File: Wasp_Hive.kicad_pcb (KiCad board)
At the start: 2 copper layers, 132.8 x 172.5 mm, 157 parts, among them J0 WASP_OUT, J1 WASP_OUT, J10 WASP_OUT, J11 WASP_OUT, J12 WASP_OUT, J13 WASP_OUT, J14 WASP_OUT, J15 WASP_OUT, J16 DENS_OUT, J17 DENS_IN, J18 DROP_OUT, J19 PANIC_IN, J2 WASP_OUT, J20 GND, J21 GND, J22 GND, J23 GND, J24 GND, J25 PWR, J26 GND, J27 GND, J3 WASP_OUT, J4 WASP_OUT, J5 WASP_OUT, J6 WASP_OUT, J7 WASP_OUT, J8 WASP_OUT, J9 WASP_OUT, Q1 MMBT3904, Q2 MMBT3904, SW1 SW_SPDT, U0 74HC245, U1 74HC245, U2 MCP6002-xP, U3 MCP6002-xP, U4 TEENSY_3.2_MINIMAL, U5 L78M05ABDT-TR

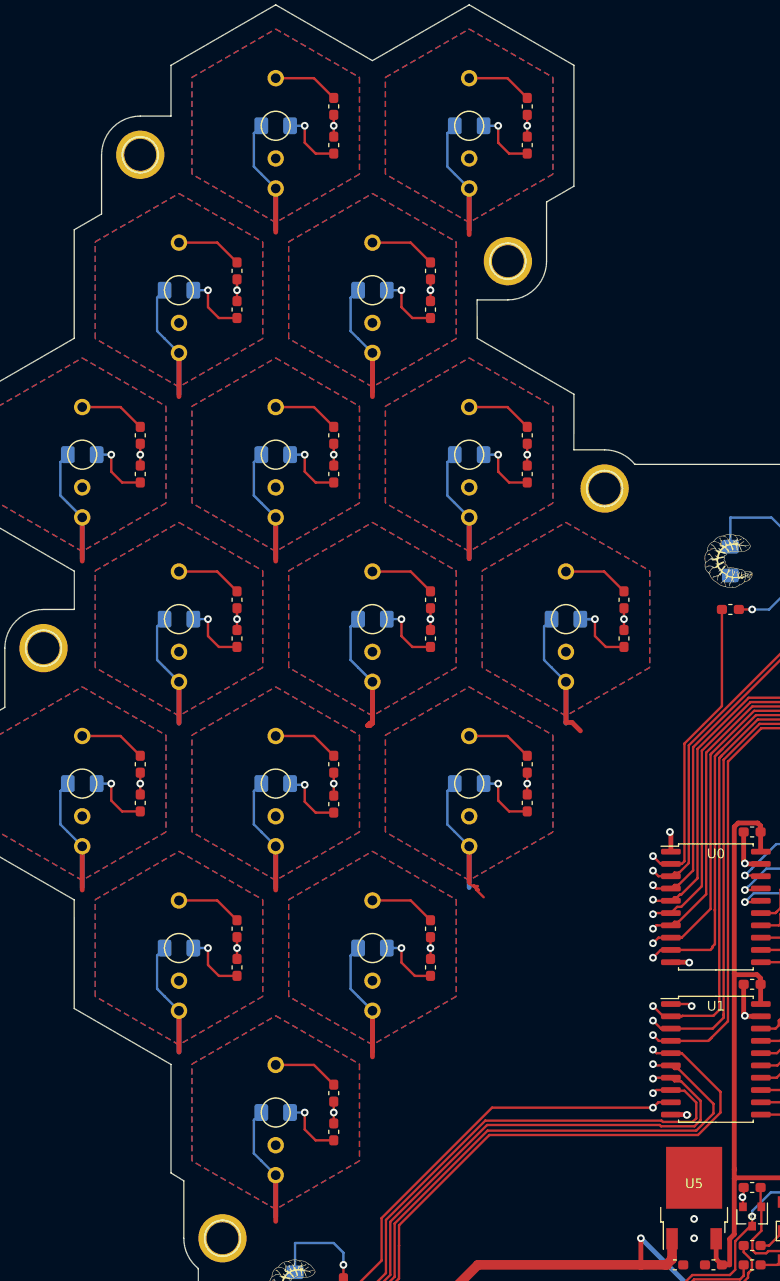
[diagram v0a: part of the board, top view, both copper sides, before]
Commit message: not working
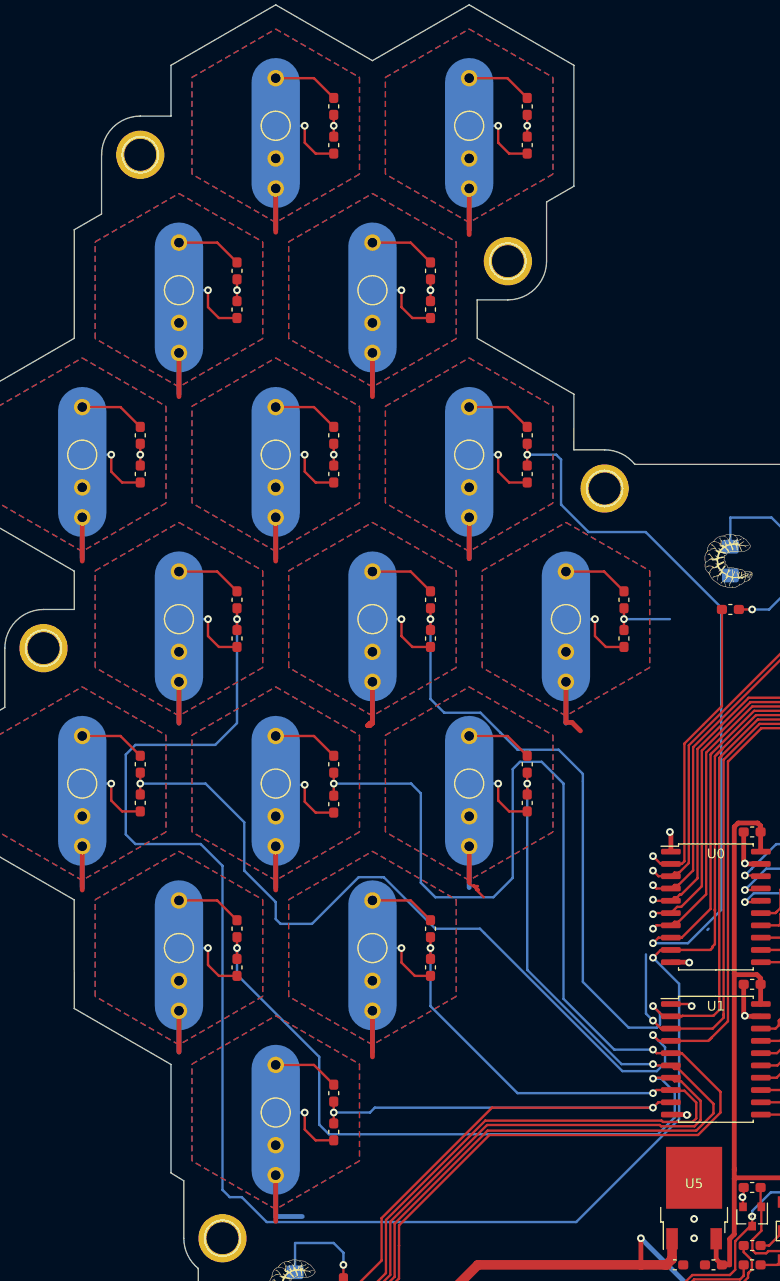
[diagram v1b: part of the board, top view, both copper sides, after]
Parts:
- J0, J1, J10, J11, J12, J13, J14, J15, J2, J3, J4, J5, J6, J7, J8, J9: footprint HammerheadAudio:EuroJack_Hex_SmallHoles_NoSilk_Clearance -> HammerheadAudio:EuroJack_Hex_SmallHoles_NoSilk_Clearance2
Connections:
- J0 pad 3: (no net) -> Net-(J0-Pad3)
- J1 pad 3: (no net) -> Net-(J1-Pad3)
- J10 pad 3: (no net) -> Net-(J10-Pad3)
- J11 pad 3: (no net) -> Net-(J11-Pad3)
- J12 pad 3: (no net) -> Net-(J12-Pad3)
- J13 pad 3: (no net) -> Net-(J13-Pad3)
- J14 pad 3: (no net) -> Net-(J14-Pad3)
- J15 pad 3: (no net) -> Net-(J15-Pad3)
- J2 pad 3: (no net) -> Net-(J2-Pad3)
- J3 pad 3: (no net) -> Net-(J3-Pad3)
- J4 pad 3: (no net) -> Net-(J4-Pad3)
- J5 pad 3: (no net) -> Net-(J5-Pad3)
- J6 pad 3: (no net) -> Net-(J6-Pad3)
- J7 pad 3: (no net) -> Net-(J7-Pad3)
- J8 pad 3: (no net) -> Net-(J8-Pad3)
- J9 pad 3: (no net) -> Net-(J9-Pad3)
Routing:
- net O7: track 127.5 -> 275.0 mm
- net O11: track 123.1 -> 204.2 mm
- net O10: track 180.8 -> 259.0 mm
- net O6: track 109.5 -> 178.6 mm
- net O13: track 90.1 -> 155.2 mm
- net O8: track 148.2 -> 209.2 mm
- net O12: track 106.3 -> 142.5 mm
- net O15: track 47.4 -> 80.6 mm
- net O14: track 70.1 -> 102.8 mm
- net O9: track 166.3 -> 178.4 mm
- net GND: track 306.0 -> 308.7 mm
